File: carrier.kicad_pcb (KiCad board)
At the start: 2 copper layers, 50 x 50 mm, 97 parts, among them J1 732511151, J2 732511151, J3 732511151, J4 732511151, J5 FTSH-105-01-L-DV-K, J6 USB4110-GF-A, J7 732511151, J8 732511151, J9 M20-9990445, U2 STM32C071G8Ux, Y2 38.4MHz

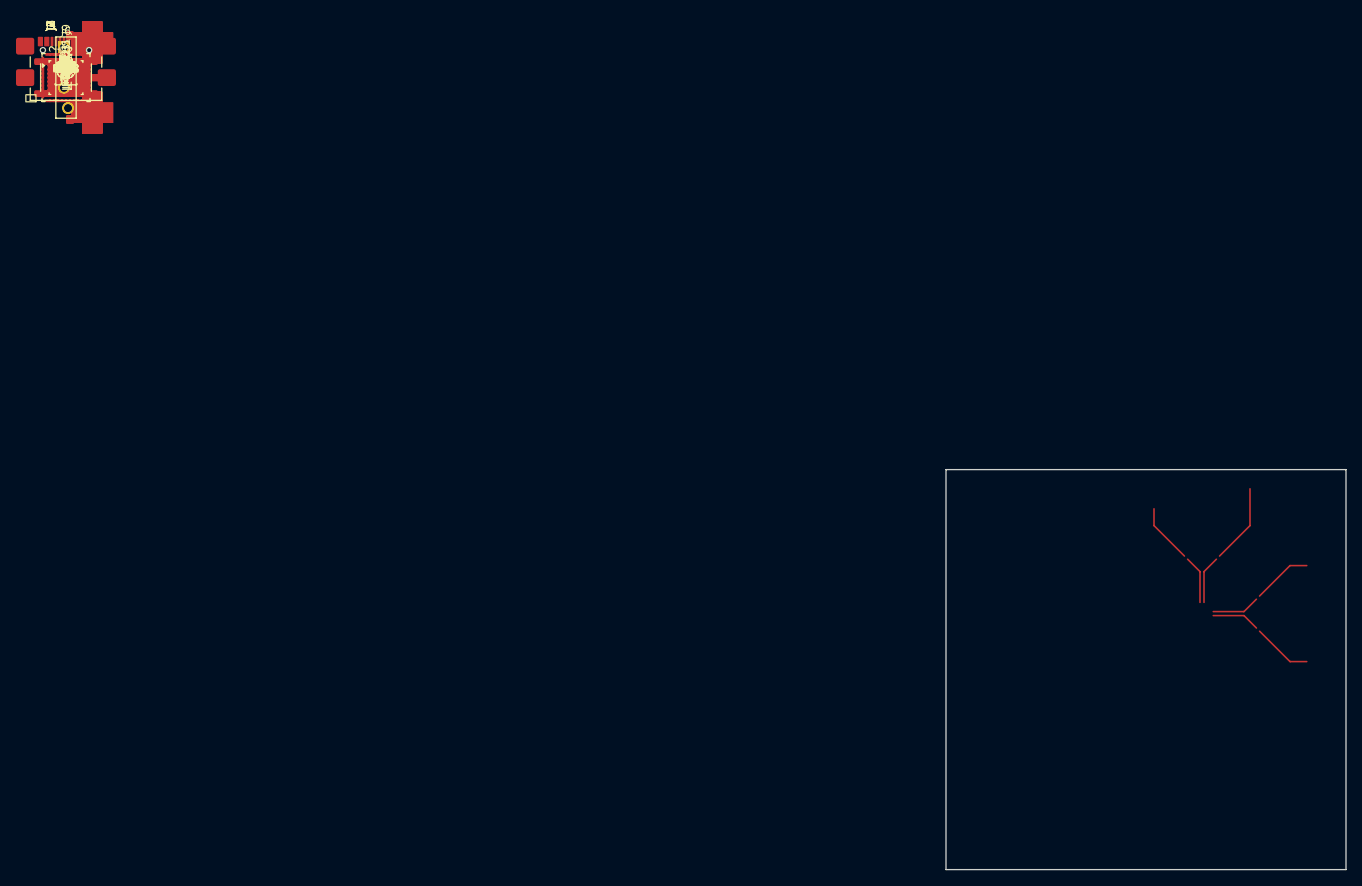
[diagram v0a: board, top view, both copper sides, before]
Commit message: layout complete
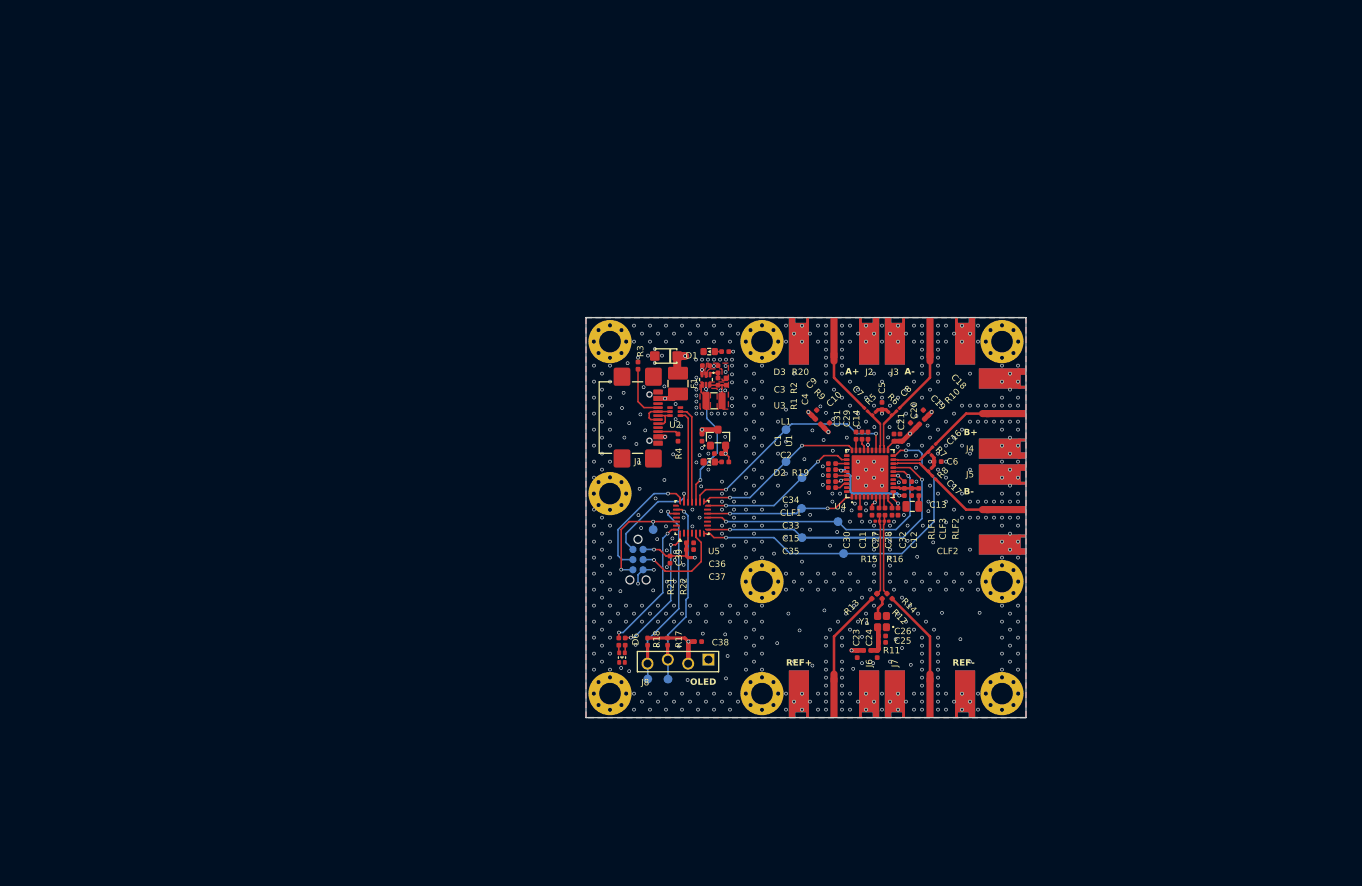
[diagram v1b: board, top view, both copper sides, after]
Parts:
- removed C22: 100nF, ar_passives:C_0402
- removed C40: 1uF, ar_passives:C_0402
- removed D4: Red, ar_opto:LED_0603
- removed D5: ~, ar_discrete:SOD123W
- removed J9: M20-9990445, ar_connector:Header 2.54 1x04 Staggered
- removed RLF3: TBD, ar_passives:R_0402
- removed TP2: MUX, ar_non-bom:Testpad_1mm
- removed U6: ~, ar_ic:SOT563
- removed Y2: 38.4MHz, ar_passives:XTAL2016-4
- added C38: 1uF, ar_passives:C_0402, F.Cu at (79.0, 70.5)
- added C5: 100nF, ar_passives:C_0402, F.Cu at (102.0, 41.0)
- added C6: 100nF, ar_passives:C_0402, F.Cu at (109.0, 48.0)
- added D6: RG, ar_opto:APHB1608GR, F.Cu at (69.5, 72.5)
- added H1: GND, MountingHole:MountingHole_2.7mm_M2.5_Pad_Via, F.Cu at (87.0, 33.0)
- added H2: GND, MountingHole:MountingHole_2.7mm_M2.5_Pad_Via, F.Cu at (117.0, 33.0)
- added H3: GND, MountingHole:MountingHole_2.7mm_M2.5_Pad_Via, F.Cu at (87.0, 77.0)
- added H4: GND, MountingHole:MountingHole_2.7mm_M2.5_Pad_Via, F.Cu at (117.0, 77.0)
- added H5: GND, MountingHole:MountingHole_2.7mm_M2.5_Pad_Via, F.Cu at (117.0, 63.0)
- added H6: GND, MountingHole:MountingHole_2.7mm_M2.5_Pad_Via, F.Cu at (87.0, 63.0)
- added H7: GND, MountingHole:MountingHole_2.7mm_M2.5_Pad_Via, F.Cu at (68.0, 33.0)
- added H8: GND, MountingHole:MountingHole_2.7mm_M2.5_Pad_Via, F.Cu at (68.0, 77.0)
- added H9: GND, MountingHole:MountingHole_2.7mm_M2.5_Pad_Via, F.Cu at (68.0, 52.0)
- added J10: TC2030-NL-FP, ar_connector:TC2030-xxx-NL, B.Cu at (71.5, 60.2)
- added RLF1: TBD, ar_passives:R_0402, F.Cu at (104.8, 51.8)
- added U5: STM32C071G8Ux, Package_DFN_QFN:QFN-28_4x4mm_P0.5mm, F.Cu at (78.2, 55.0)
- added Y1: 38.4MHz, ar_passives:XTAL2016-4, F.Cu at (102.0, 68.0)
- C1, C10, C2, C23, C24: value 100nF -> 10uF
- C12, C37, C39: value 1uF -> 100nF
- C15, C36: value 100nF -> 1uF
- C18, C19: value 22pF -> 10uF; footprint ar_passives:C_0201 -> ar_passives:C_0402
- C25: value 10uF -> 1uF
- C26, C27, C28: value 10uF -> 100nF; footprint ar_passives:C_0805 -> ar_passives:C_0402
- C29, C30, C31, C33: footprint ar_passives:C_0805 -> ar_passives:C_0402
- C32, C35: value 10uF -> 1uF; footprint ar_passives:C_0805 -> ar_passives:C_0402
- C34: value 1uF -> 10uF
- C7: value 1uF -> 22pF; footprint ar_passives:C_0402 -> ar_passives:C_0201
- C8: value 10uF -> 22pF; footprint ar_passives:C_0402 -> ar_passives:C_0201
- CLF1: footprint ar_passives:C_0603 -> ar_passives:C_0402
- CLF2: value 0pF -> 10nF; footprint ar_passives:C_0402 -> ar_passives:C_0805
- D1: value Green -> ~; footprint ar_opto:LED_0603 -> ar_discrete:SOD123W
- J1: value 732511151 -> USB4110-GF-A; footprint ar_connector:Molex 73251-1151 -> ar_connector:USB-C USB4110
- J5: value FTSH-105-01-L-DV-K -> 732511151; footprint ar_connector:FTSH-105-01-X-DV-K -> ar_connector:Molex 73251-1151
- J6: value USB4110-GF-A -> 732511151; footprint ar_connector:USB-C USB4110 -> ar_connector:Molex 73251-1151
- J8: value 732511151 -> M20-9990445; footprint ar_connector:Molex 73251-1151 -> ar_connector:Header 2.54 1x04 Staggered
- R1: value 0R -> 200k
- R10: value 44.2k -> 0R
- R11, R12, R13, R14: value 1k -> 0R
- R15, R16: value 5.11k -> 51R; footprint ar_passives:R_0402 -> ar_passives:R_0201
- R17, R18, R3: value 0R -> 5.11k
- R19, R20: value 0R -> 1k
- R2: value 51R -> 44.2k; footprint ar_passives:R_0201 -> ar_passives:R_0402
- R21, R22: value 5.11k -> 1k
- R4: value 51R -> 5.11k; footprint ar_passives:R_0201 -> ar_passives:R_0402
- R9: value 200k -> 0R
- TP1: value SCK -> SDA
- TP10: value SDA -> CE
- TP11: value SDA -> CS
- TP3: value SDI -> SDA
- TP4: value RC -> SCL
- TP5: value RD -> SCK
- TP6: value CE -> MUX
- TP7: value CS -> SDI
- TP8: value SCL -> RC
- TP9: value SDA -> RD
- U1: footprint ar_ic:QFN40 -> ar_ic:SOT-23-3
- U2: value STM32C071G8Ux -> ~; footprint Package_DFN_QFN:QFN-28_4x4mm_P0.5mm -> ar_ic:DFN6-1.55x1.75
- U3: footprint ar_ic:SOT-23-3 -> ar_ic:SOT563
- U4: footprint ar_ic:DFN6-1.55x1.75 -> ar_ic:QFN40
- moved J7 134.4 mm to (108.0, 80.0), turned to 90 degrees
- moved J5 131.6 mm to (120.0, 54.0), turned to 180 degrees
- moved J4 127.1 mm to (120.0, 42.0), turned to 180 degrees
- moved J6 125.0 mm to (96.0, 80.0), turned to 90 degrees
- moved C24 124.4 mm to (101.4, 72.0), turned to -90 degrees
- moved C25 124.0 mm to (102.0, 70.6)
- moved C26 123.6 mm to (102.0, 69.8)
- moved R11 123.1 mm to (100.2, 71.6)
- moved C23 122.4 mm to (98.9, 72.0), turned to -90 degrees
- moved R14 121.7 mm to (103.0, 64.8), turned to 135 degrees
- moved R12 120.6 mm to (101.7, 64.8), turned to 135 degrees
- moved R13 120.1 mm to (101.0, 64.8), turned to 45 degrees
- moved C17 119.5 mm to (108.5, 50.0), turned to -45 degrees
- moved CLF2 118.6 mm to (105.8, 53.6), turned to 180 degrees
- moved R8 118.6 mm to (108.0, 49.0), turned to -135 degrees
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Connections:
- C1 pad 1: /REF_P -> VBUS
- C1 pad 2: /OSC_P -> GND
- C15 pad 1: 3V3_BUF -> 3V3_SYN
- C16 pad 1: /RF_A_P -> /RF_B_P
- C16 pad 2: /SMA_A_P -> /SMA_B_P
- C17 pad 1: /RF_A_N -> /RF_B_N
- C17 pad 2: /SMA_A_N -> /SMA_B_N
- C18 pad 1: /RF_B_P -> 3V3_BUCK
- C18 pad 2: /SMA_B_P -> GND
- C19 pad 1: /RF_B_N -> 3V3_BUF
- C19 pad 2: /SMA_B_N -> GND
- C2 pad 1: /REF_N -> 3V3_MCU
- C2 pad 2: /OSC_N -> GND
- C20 pad 1: 3V3_MCU -> 3V3_BUF
- C21 pad 1: 3V3_MCU -> 3V3_BUF
- C23 pad 1: 3V3_BUF -> 3V3_MCU
- C24 pad 1: 3V3_BUF -> 3V3_OSC
- C25 pad 1: /VbiasVCO2 -> 3V3_OSC
- C26 pad 1: 3V3_BUCK -> 3V3_OSC
- C27 pad 1: VBUS -> /REF_P
- C27 pad 2: GND -> /OSC_P
- C28 pad 1: 3V3_BUCK -> /REF_N
- C28 pad 2: GND -> /OSC_N
- C29 pad 1: 3V3_BUCK -> /VbiasVCO2
- C3 pad 1: /VrefVCO -> VBUS
- C30 pad 1: 3V3_BUCK -> /VbiasVCO
- C31 pad 1: VBUS -> /VrefVCO2
- C32 pad 1: 3V3_MCU -> /VregIN
- C33 pad 1: 3V3_BUF -> /VrefVCO
- C34 pad 1: /VregVCO -> /VbiasVARAC
- C35 pad 1: 3V3_OSC -> /VregVCO
- C36 pad 1: 3V3_OSC -> 3V3_MCU
- C39 pad 1: 3V3_BUF -> 3V3_MCU
- C4 pad 1: /VbiasVARAC -> 3V3_BUCK
- C7 pad 1: /VregIN -> /RF_A_P
- C7 pad 2: GND -> /SMA_A_P
- C8 pad 1: /VrefVCO2 -> /RF_A_N
- C8 pad 2: GND -> /SMA_A_N
- C9 pad 1: /VbiasVCO -> 3V3_BUCK
- CLF1 pad 1: /CPOut -> GND
- CLF1 pad 2: GND -> /VTUNE
- CLF3 pad 1: GND -> /CPOut
- CLF3 pad 2: /VTUNE -> GND
- D1 pad A: Net-(D1-PadA) -> GND
- D1 pad K: GND -> VBUS
- J2 pad inner: /SMA_A_N -> /SMA_A_P
- J3 pad inner: /SMA_B_P -> /SMA_A_N
- J4 pad inner: /SMA_B_N -> /SMA_B_P
- L1 pad 1: Net-(U6-SW) -> Net-(U3-SW)
- R1 pad 2: 3V3_SYN -> Net-(U3-FB)
- R10 pad 1: Net-(U6-FB) -> 3V3_BUCK
- R10 pad 2: GND -> 3V3_BUF
- R11 pad 2: Net-(D1-PadA) -> 3V3_OSC
- R12 pad 1: 3V3_BUCK -> /REF_TCXO
- R12 pad 2: Net-(D2-PadA) -> /REF_P
- R13 pad 1: /LED_STAT -> /REF_SMA_P
- R13 pad 2: Net-(D3-PadA) -> /REF_P
- R14 pad 1: /LED_ERR -> /REF_SMA_N
- R14 pad 2: Net-(D4-PadA) -> /REF_N
- R15 pad 1: Net-(J6-CC1) -> /REF_P
- R16 pad 1: Net-(J6-CC2) -> /REF_N
- R17 pad 1: 3V3_BUCK -> 3V3_MCU
- R17 pad 2: 3V3_OSC -> /OLED_SCL
- R18 pad 1: /REF_TCXO -> 3V3_MCU
- R18 pad 2: /REF_P -> /OLED_SDA
- R19 pad 1: /REF_SMA_N -> 3V3_MCU
- R19 pad 2: /REF_N -> Net-(D2-PadA)
- R2 pad 1: 3V3_BUF -> Net-(U3-FB)
- R2 pad 2: /RF_A_P -> GND
- R20 pad 1: /REF_SMA_P -> 3V3_BUCK
- R20 pad 2: /REF_P -> Net-(D3-PadA)
- R21 pad 1: 3V3_MCU -> /LED_STAT
- R21 pad 2: /OLED_SDA -> Net-(D6A-Red_A)
- R22 pad 1: 3V3_MCU -> /LED_ERR
- R22 pad 2: /OLED_SCL -> Net-(D6B-Green_A)
- R3 pad 1: 3V3_BUCK -> Net-(J1-CC1)
- R3 pad 2: 3V3_BUF -> GND
- R4 pad 1: 3V3_BUF -> Net-(J1-CC2)
- R4 pad 2: /RF_A_N -> GND
- R5 pad 2: /RF_B_P -> /RF_A_P
- R6 pad 2: /RF_B_N -> /RF_A_N
- R7 pad 1: /REF_P -> 3V3_BUF
- R7 pad 2: GND -> /RF_B_P
- R8 pad 1: /REF_N -> 3V3_BUF
- R8 pad 2: GND -> /RF_B_N
- R9 pad 2: Net-(U6-FB) -> 3V3_SYN
- TP1 pad 1: /SYN.SCK -> /DBG_TX
- TP10 pad 1: /DBG_RX -> /SYN.CE
- TP11 pad 1: /DBG_TX -> /SYN.~{CS}
- TP3 pad 1: /SYN.SDI -> /OLED_SCL
- TP4 pad 1: /SYN.RC -> /OLED_SDA
- TP5 pad 1: /SYN.RD -> /SYN.SCK
- TP6 pad 1: /SYN.CE -> /SYN.MUX
- TP7 pad 1: /SYN.~{CS} -> /SYN.SDI
- TP8 pad 1: /OLED_SCL -> /SYN.RD
- TP9 pad 1: /OLED_SDA -> /SYN.RC
- U1 pad 1: /SYN.CE -> GND
- U1 pad 2: GND -> 3V3_MCU
- U1 pad 3: /VbiasVCO -> VBUS
- U2 pad 1: /MCU_REF_IN -> /USB_DP
- U2 pad 2: unconnected-(U2-PC15-Pad2) -> /USB_DN
- U2 pad 3: 3V3_MCU -> GND
- U2 pad 4: GND -> unconnected-(U2-NC-Pad4)
- U2 pad 5: /~{DBG_NRST} -> /CON_DN
- U2 pad 6: /DBG_TX -> /CON_DP
- U3 pad 1: GND -> Net-(U3-FB)
- U3 pad 2: 3V3_MCU -> GND
- U4 pad 1: /USB_DN -> /SYN.CE
- U4 pad 2: /USB_DP -> GND
- U4 pad 3: GND -> /VbiasVCO
- U4 pad 4: unconnected-(U4-NC-Pad4) -> GND
- U4 pad 5: /CON_DP -> unconnected-(U4-NC-Pad5)
- U4 pad 6: /CON_DN -> GND
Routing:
- net 3V3_MCU: track 0.00 -> 71.1 mm, vias 0 -> 5
- net /SYN.SDI: track 0.00 -> 47.2 mm, vias 0 -> 2
- net /SYN.MUX: track 0.00 -> 44.6 mm, vias 0 -> 2
- net 3V3_BUCK: track 0.00 -> 44.3 mm, vias 0 -> 5
- net /SYN.SCK: track 0.00 -> 33.8 mm, vias 0 -> 2
- net /SYN.~{CS}: track 0.00 -> 29.1 mm, vias 0 -> 2
- net /OLED_SDA: track 0.00 -> 26.6 mm, vias 0 -> 1
- net /OLED_SCL: track 0.00 -> 25.1 mm, vias 0 -> 1
- net /SYN.RC: track 0.00 -> 21.8 mm, vias 0 -> 2
- net 3V3_BUF: track 0.00 -> 21.4 mm, vias 0 -> 3
- net /SYN.RD: track 0.00 -> 20.1 mm, vias 0 -> 2
- net VBUS: track 0.00 -> 20.1 mm, vias 0 -> 3
- net /SYN.CE: track 0.00 -> 18.9 mm, vias 0 -> 2
- net /LED_STAT: track 0.00 -> 17.1 mm, vias 0 -> 2
- net /LED_ERR: track 0.00 -> 17.1 mm, vias 0 -> 2
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- added copper zone on F.Cu, net 3V3_BUCK
- added copper zone on In2.Cu, net 3V3_SYN
- added copper zone on B.Cu, net GND
- added copper zone on F.Cu, net GND
- added copper zone on In1.Cu, net GND
- added copper zone on In2.Cu, net GND
- added copper zone on F.Cu, net Net-(U3-SW)
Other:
- board size 50 x 50 mm -> 55 x 50 mm
- copper layers 2 -> 4
- board text added: "A+"
- board text added: "A-"
- board text added: "B+"
- board text added: "B-"
- board text added: "OLED"
- board text added: "REF+"
- board text added: "REF-"
